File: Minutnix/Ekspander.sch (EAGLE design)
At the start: 14 parts, among them X1 FH12-12S-0.5S_THINNER, X6 JST-XH-03-PIN-LONG-PAD

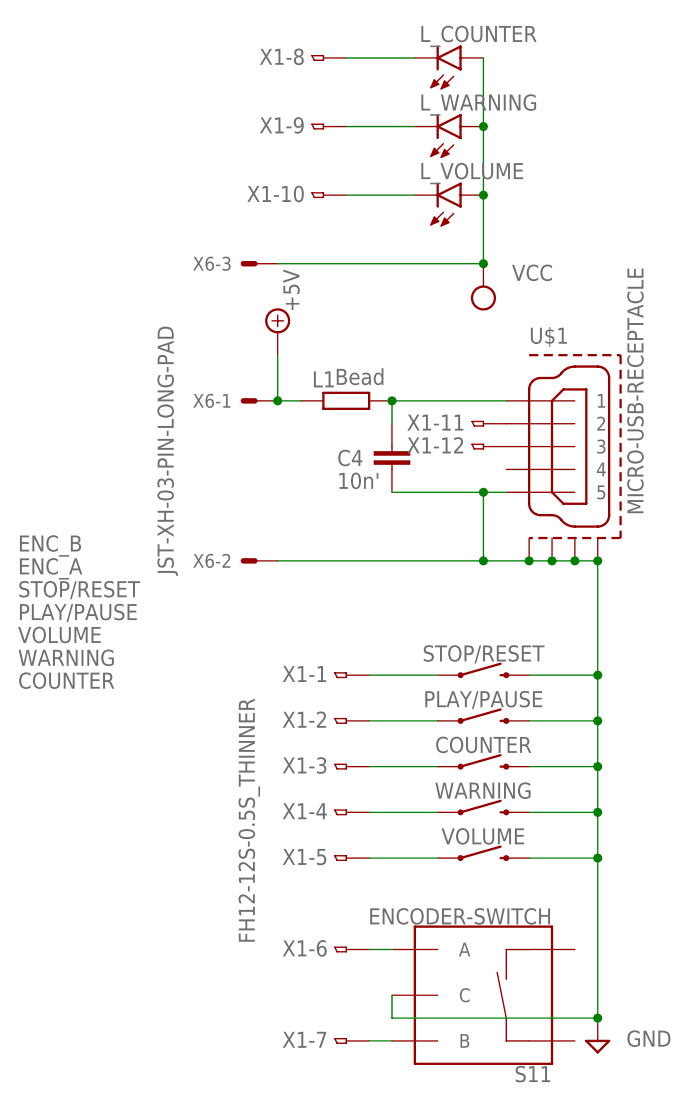
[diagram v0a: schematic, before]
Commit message: Probably final routing of Expander board
DRC 8mils clean
libs actualisation
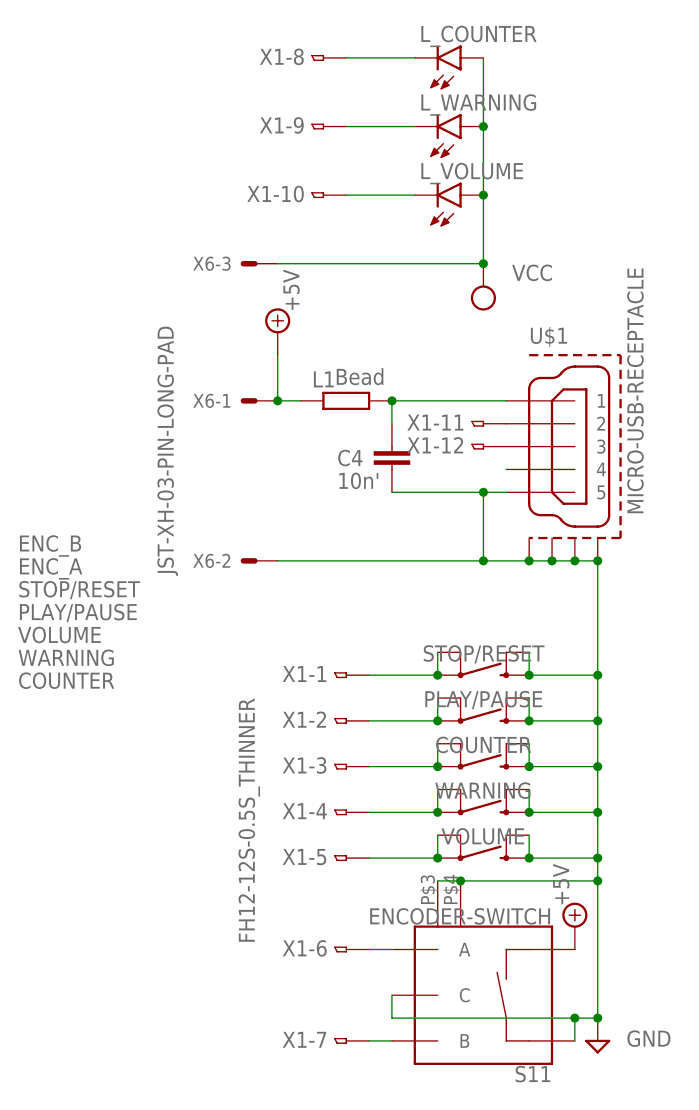
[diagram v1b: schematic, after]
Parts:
- COUNTER, PLAY/PAUSE, STOP/RESET, VOLUME, WARNING: device SparkFun-Switches:MOMENTARY-SWITCH-SPST-PTH-12MM -> MySparkFun-Switches:MOMENTARY-SWITCH-SPST-PTH-12MM
- S11: device SparkFun-Switches:ENCODER-SWITCH -> MySparkFun-Switches:ENCODER-SWITCH
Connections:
- net +5V: now also S11.SW-
- net GND: now also COUNTER.4, PLAY/PAUSE.4, S11.GND1, S11.GND2, S11.SW+, STOP/RESET.4, VOLUME.4, WARNING.4
- net N$2: now also STOP/RESET.3
- net N$3: now also PLAY/PAUSE.3
- net N$4: now also COUNTER.3
- net N$5: now also WARNING.3
- net N$6: now also VOLUME.3
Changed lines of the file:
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@@
 </classes>
 <parts>
-<part name="S11" library="SparkFun-Switches" library_urn="urn:adsk.eagle:library:535" deviceset="ENCODER-SWITCH" device="" package3d_urn="urn:adsk.eagle:package:40158/1"/>
+<part name="S11" library="MySparkFun-Switches" deviceset="ENCODER-SWITCH" device="" package3d_urn="urn:adsk.eagle:package:40158/1"/>
 <part name="L_WARNING" library="led" library_urn="urn:adsk.eagle:library:259" deviceset="LED" device="CHIPLED_0805" package3d_urn="urn:adsk.eagle:package:15821/2"/>
 <part name="X1" library="My_con-hirose" deviceset="FH12-12S-0.5S_THINNER" device=""/>
@@
 <part name="L1" library="rcl" library_urn="urn:adsk.eagle:library:334" deviceset="R-EU_" device="R0603" package3d_urn="urn:adsk.eagle:package:23555/3" value="Bead"/>
 <part name="C4" library="rcl" library_urn="urn:adsk.eagle:library:334" deviceset="C-EU" device="C0603" package3d_urn="urn:adsk.eagle:package:23616/2" value="10n'"/>
-<part name="COUNTER" library="SparkFun-Switches" library_urn="urn:adsk.eagle:library:535" deviceset="MOMENTARY-SWITCH-SPST" device="-PTH-12MM" package3d_urn="urn:adsk.eagle:package:40164/1"/>
-<part name="WARNING" library="SparkFun-Switches" library_urn="urn:adsk.eagle:library:535" deviceset="MOMENTARY-SWITCH-SPST" device="-PTH-12MM" package3d_urn="urn:adsk.eagle:package:40164/1"/>
-<part name="VOLUME" library="SparkFun-Switches" library_urn="urn:adsk.eagle:library:535" deviceset="MOMENTARY-SWITCH-SPST" device="-PTH-12MM" package3d_urn="urn:adsk.eagle:package:40164/1"/>
-<part name="PLAY/PAUSE" library="SparkFun-Switches" library_urn="urn:adsk.eagle:library:535" deviceset="MOMENTARY-SWITCH-SPST" device="-PTH-12MM" package3d_urn="urn:adsk.eagle:package:40164/1"/>
-<part name="STOP/RESET" library="SparkFun-Switches" library_urn="urn:adsk.eagle:library:535" deviceset="MOMENTARY-SWITCH-SPST" device="-PTH-12MM" package3d_urn="urn:adsk.eagle:package:40164/1"/>
+<part name="COUNTER" library="MySparkFun-Switches" deviceset="MOMENTARY-SWITCH-SPST" device="-PTH-12MM" package3d_urn="urn:adsk.eagle:package:40164/1"/>
+<part name="WARNING" library="MySparkFun-Switches" deviceset="MOMENTARY-SWITCH-SPST" device="-PTH-12MM" package3d_urn="urn:adsk.eagle:package:40164/1"/>
+<part name="VOLUME" library="MySparkFun-Switches" deviceset="MOMENTARY-SWITCH-SPST" device="-PTH-12MM" package3d_urn="urn:adsk.eagle:package:40164/1"/>
+<part name="PLAY/PAUSE" library="MySparkFun-Switches" deviceset="MOMENTARY-SWITCH-SPST" device="-PTH-12MM" package3d_urn="urn:adsk.eagle:package:40164/1"/>
+<part name="STOP/RESET" library="MySparkFun-Switches" deviceset="MOMENTARY-SWITCH-SPST" device="-PTH-12MM" package3d_urn="urn:adsk.eagle:package:40164/1"/>
 <part name="SUPPLY20" library="supply2" library_urn="urn:adsk.eagle:library:372" deviceset="VCC" device=""/>
 <part name="U$1" library="con-molex-usb" deviceset="MICRO-USB-RECEPTACLE" device=""/>
@@
 <part name="L_COUNTER" library="led" library_urn="urn:adsk.eagle:library:259" deviceset="LED" device="CHIPLED_0805" package3d_urn="urn:adsk.eagle:package:15821/2"/>
 <part name="L_VOLUME" library="led" library_urn="urn:adsk.eagle:library:259" deviceset="LED" device="CHIPLED_0805" package3d_urn="urn:adsk.eagle:package:15821/2"/>
+<part name="SUPPLY2" library="supply2" library_urn="urn:adsk.eagle:library:372" deviceset="+5V" device=""/>
 </parts>
 <sheets>
@@
 <attribute name="VALUE" x="74.168" y="196.215" size="1.778" layer="96" rot="MR180"/>
 </instance>
+<instance part="SUPPLY2" gate="+5V" x="91.44" y="109.22" smashed="yes" rot="MR0">
+<attribute name="VALUE" x="90.805" y="116.205" size="1.778" layer="96" rot="MR270"/>
+</instance>
 </instances>
 <busses>
@@
 <junction x="58.42" y="167.64"/>
 </segment>
+<segment>
+<pinref part="SUPPLY2" gate="+5V" pin="+5V"/>
+<pinref part="S11" gate="G$1" pin="SW-"/>
+</segment>
 </net>
 <net name="GND" class="0">
@@
 <wire x1="93.98" y1="127" x2="93.98" y2="121.92" width="0.1524" layer="91"/>
 <wire x1="93.98" y1="121.92" x2="93.98" y2="116.84" width="0.1524" layer="91"/>
-<wire x1="93.98" y1="116.84" x2="93.98" y2="99.06" width="0.1524" layer="91"/>
-<wire x1="71.12" y1="99.06" x2="93.98" y2="99.06" width="0.1524" layer="91"/>
+<wire x1="93.98" y1="116.84" x2="93.98" y2="114.3" width="0.1524" layer="91"/>
+<wire x1="93.98" y1="114.3" x2="93.98" y2="99.06" width="0.1524" layer="91"/>
+<wire x1="71.12" y1="99.06" x2="91.44" y2="99.06" width="0.1524" layer="91"/>
 <pinref part="S11" gate="G$1" pin="C"/>
+<wire x1="91.44" y1="99.06" x2="93.98" y2="99.06" width="0.1524" layer="91"/>
 <wire x1="71.12" y1="101.6" x2="71.12" y2="99.06" width="0.1524" layer="91"/>
 <pinref part="SUPPLY1" gate="GND" pin="GND"/>
@@
 <wire x1="86.36" y1="132.08" x2="93.98" y2="132.08" width="0.1524" layer="91"/>
 <junction x="93.98" y="132.08"/>
+<pinref part="S11" gate="G$1" pin="GND1"/>
+<wire x1="76.2" y1="114.3" x2="78.74" y2="114.3" width="0.1524" layer="91"/>
+<junction x="93.98" y="114.3"/>
+<pinref part="S11" gate="G$1" pin="GND2"/>
+<wire x1="78.74" y1="114.3" x2="93.98" y2="114.3" width="0.1524" layer="91"/>
+<junction x="78.74" y="114.3"/>
+<pinref part="VOLUME" gate="G$1" pin="4"/>
+<wire x1="86.36" y1="119.38" x2="86.36" y2="116.84" width="0.1524" layer="91"/>
+<junction x="86.36" y="116.84"/>
+<pinref part="WARNING" gate="G$1" pin="4"/>
+<wire x1="86.36" y1="124.46" x2="86.36" y2="121.92" width="0.1524" layer="91"/>
+<junction x="86.36" y="121.92"/>
+<pinref part="COUNTER" gate="G$1" pin="4"/>
+<wire x1="86.36" y1="129.54" x2="86.36" y2="127" width="0.1524" layer="91"/>
+<junction x="86.36" y="127"/>
+<pinref part="PLAY/PAUSE" gate="G$1" pin="4"/>
+<wire x1="86.36" y1="134.62" x2="86.36" y2="132.08" width="0.1524" layer="91"/>
+<junction x="86.36" y="132.08"/>
+<pinref part="STOP/RESET" gate="G$1" pin="4"/>
+<wire x1="86.36" y1="139.7" x2="86.36" y2="137.16" width="0.1524" layer="91"/>
+<junction x="86.36" y="137.16"/>
+<pinref part="S11" gate="G$1" pin="SW+"/>
+<wire x1="91.44" y1="96.52" x2="91.44" y2="99.06" width="0.1524" layer="91"/>
+<junction x="91.44" y="99.06"/>
 </segment>
 </net>
@@
 <pinref part="COUNTER" gate="G$1" pin="1"/>
 <wire x1="68.58" y1="127" x2="76.2" y2="127" width="0.1524" layer="91"/>
+<pinref part="COUNTER" gate="G$1" pin="3"/>
+<wire x1="76.2" y1="129.54" x2="76.2" y2="127" width="0.1524" layer="91"/>
+<junction x="76.2" y="127"/>
 </segment>
 </net>
@@
 <pinref part="WARNING" gate="G$1" pin="1"/>
 <wire x1="68.58" y1="121.92" x2="76.2" y2="121.92" width="0.1524" layer="91"/>
+<pinref part="WARNING" gate="G$1" pin="3"/>
+<wire x1="76.2" y1="124.46" x2="76.2" y2="121.92" width="0.1524" layer="91"/>
+<junction x="76.2" y="121.92"/>
 </segment>
 </net>
@@
 <pinref part="VOLUME" gate="G$1" pin="1"/>
 <wire x1="68.58" y1="116.84" x2="76.2" y2="116.84" width="0.1524" layer="91"/>
+<pinref part="VOLUME" gate="G$1" pin="3"/>
+<wire x1="76.2" y1="119.38" x2="76.2" y2="116.84" width="0.1524" layer="91"/>
+<junction x="76.2" y="116.84"/>
 </segment>
 </net>
@@
 <pinref part="STOP/RESET" gate="G$1" pin="1"/>
 <wire x1="68.58" y1="137.16" x2="76.2" y2="137.16" width="0.1524" layer="91"/>
+<pinref part="STOP/RESET" gate="G$1" pin="3"/>
+<wire x1="76.2" y1="139.7" x2="76.2" y2="137.16" width="0.1524" layer="91"/>
+<junction x="76.2" y="137.16"/>
 </segment>
 </net>
@@
 <pinref part="PLAY/PAUSE" gate="G$1" pin="1"/>
 <wire x1="68.58" y1="132.08" x2="76.2" y2="132.08" width="0.1524" layer="91"/>
-</segment>
-</net>
+<pinref part="PLAY/PAUSE" gate="G$1" pin="3"/>
+<wire x1="76.2" y1="134.62" x2="76.2" y2="132.08" width="0.1524" layer="91"/>
+<junction x="76.2" y="132.08"/>
+</segment>
+</net>
